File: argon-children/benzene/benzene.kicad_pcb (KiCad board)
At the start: 2 copper layers, 31.5 x 16.3 mm, 19 parts, among them U1 Conn1, U2 SPI FLASH, U3 Conn2, U4 LMC555

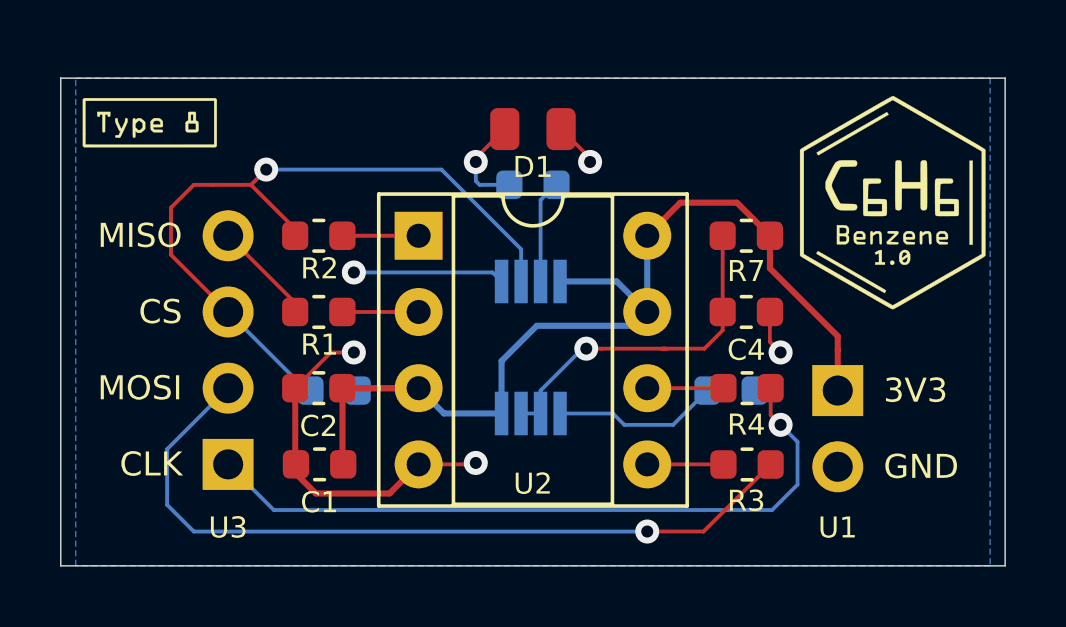
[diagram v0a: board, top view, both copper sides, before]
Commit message: 25x15 - part1
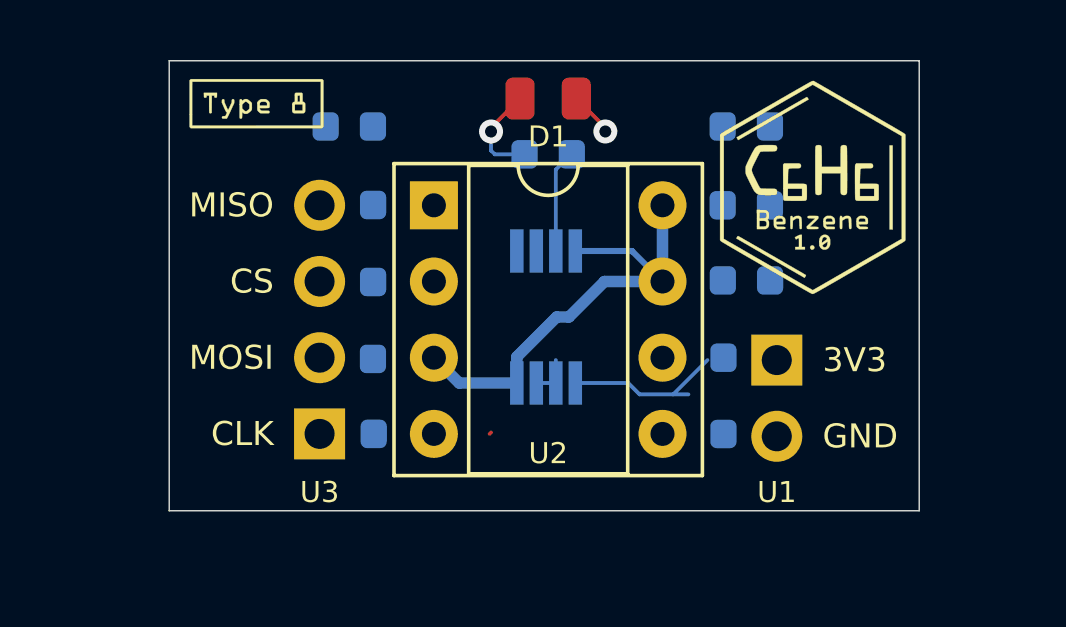
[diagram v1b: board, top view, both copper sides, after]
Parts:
- C1, C2, C4, R1, R2, R3, R4, R7: moved to B.Cu
- moved R1 6.26 mm to (97.0, 70.2)
- moved C4 6.18 mm to (110.2, 70.2)
- moved C3 3.71 mm to (110.2, 75.3)
- moved R5 3.66 mm to (97.0, 75.4)
- moved G*** 3.61 mm to (93.9, 69.4)
- moved U3 3.21 mm to (96.0, 80.4)
- moved G*** 2.71 mm to (112.5, 72.2)
- moved U1 2.27 mm to (111.3, 78.0)
- moved G*** 2.27 mm to (113.5, 70.2)
- moved R2 1.45 mm to (97.0, 72.8)
- moved C1 1.44 mm to (97.0, 80.4)
- moved C2 1.41 mm to (97.0, 77.9)
- moved D1 1.14 mm to (103.6, 69.3)
- moved U2 1.14 mm to (99.8, 72.8)
- moved U4 1.14 mm to (103.6, 76.5)
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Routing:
- net Net-(R3-Pad2): track 26.1 -> 0.00 mm, vias 1 -> 0
- net ~CS: track 24.8 -> 0.00 mm, vias 1 -> 0
- net Net-(R4-Pad2): track 23.5 -> 0.00 mm, vias 1 -> 0
- net GND: track 20.2 -> 1.56 mm, vias 5 -> 1
- net V3V3: track 34.6 -> 16.6 mm
- net Net-(C4-Pad1): track 11.6 -> 1.41 mm, vias 1 -> 0
- net Net-(R1-Pad2): track 3.47 -> 0.00 mm
- net Net-(R3-Pad1): track 2.85 -> 0.00 mm
- net Net-(R4-Pad1): track 2.62 -> 0.00 mm
- net Net-(R2-Pad1): track 2.54 -> 0.00 mm
- net Net-(R1-Pad1): track 2.54 -> 0.00 mm
- removed copper zone on B.Cu, net GND
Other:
- board size 31.5 x 16.3 mm -> 25 x 15 mm
